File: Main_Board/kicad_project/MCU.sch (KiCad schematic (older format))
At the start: 35 parts

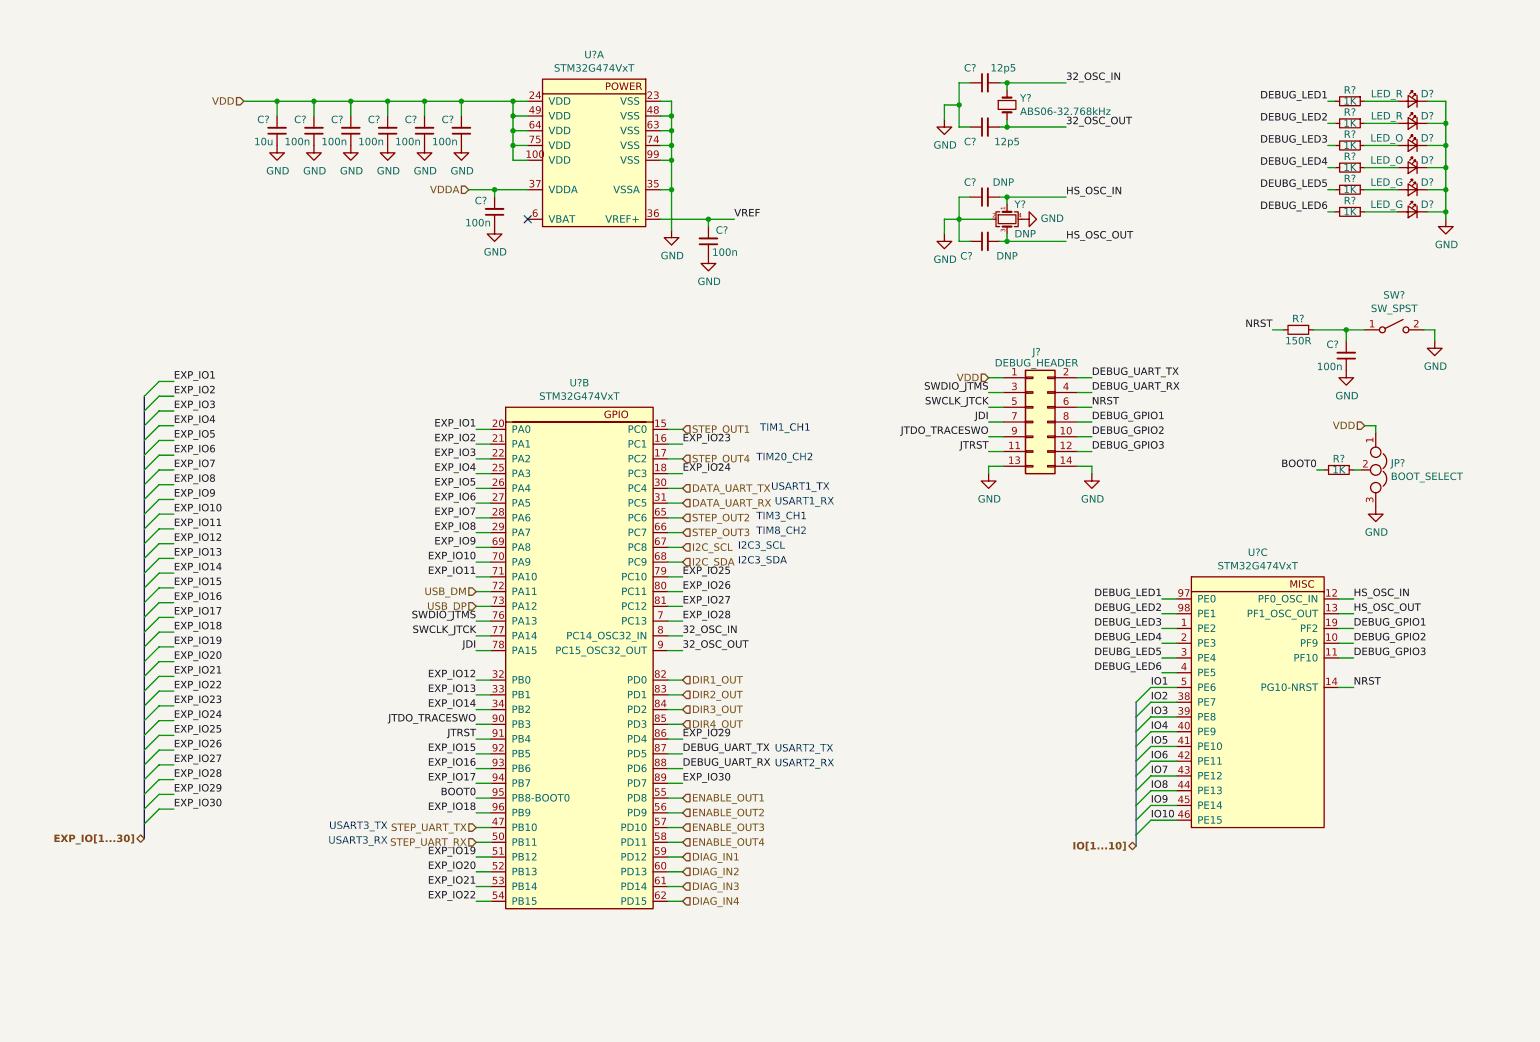
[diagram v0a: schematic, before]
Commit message: schematic rev1 finished
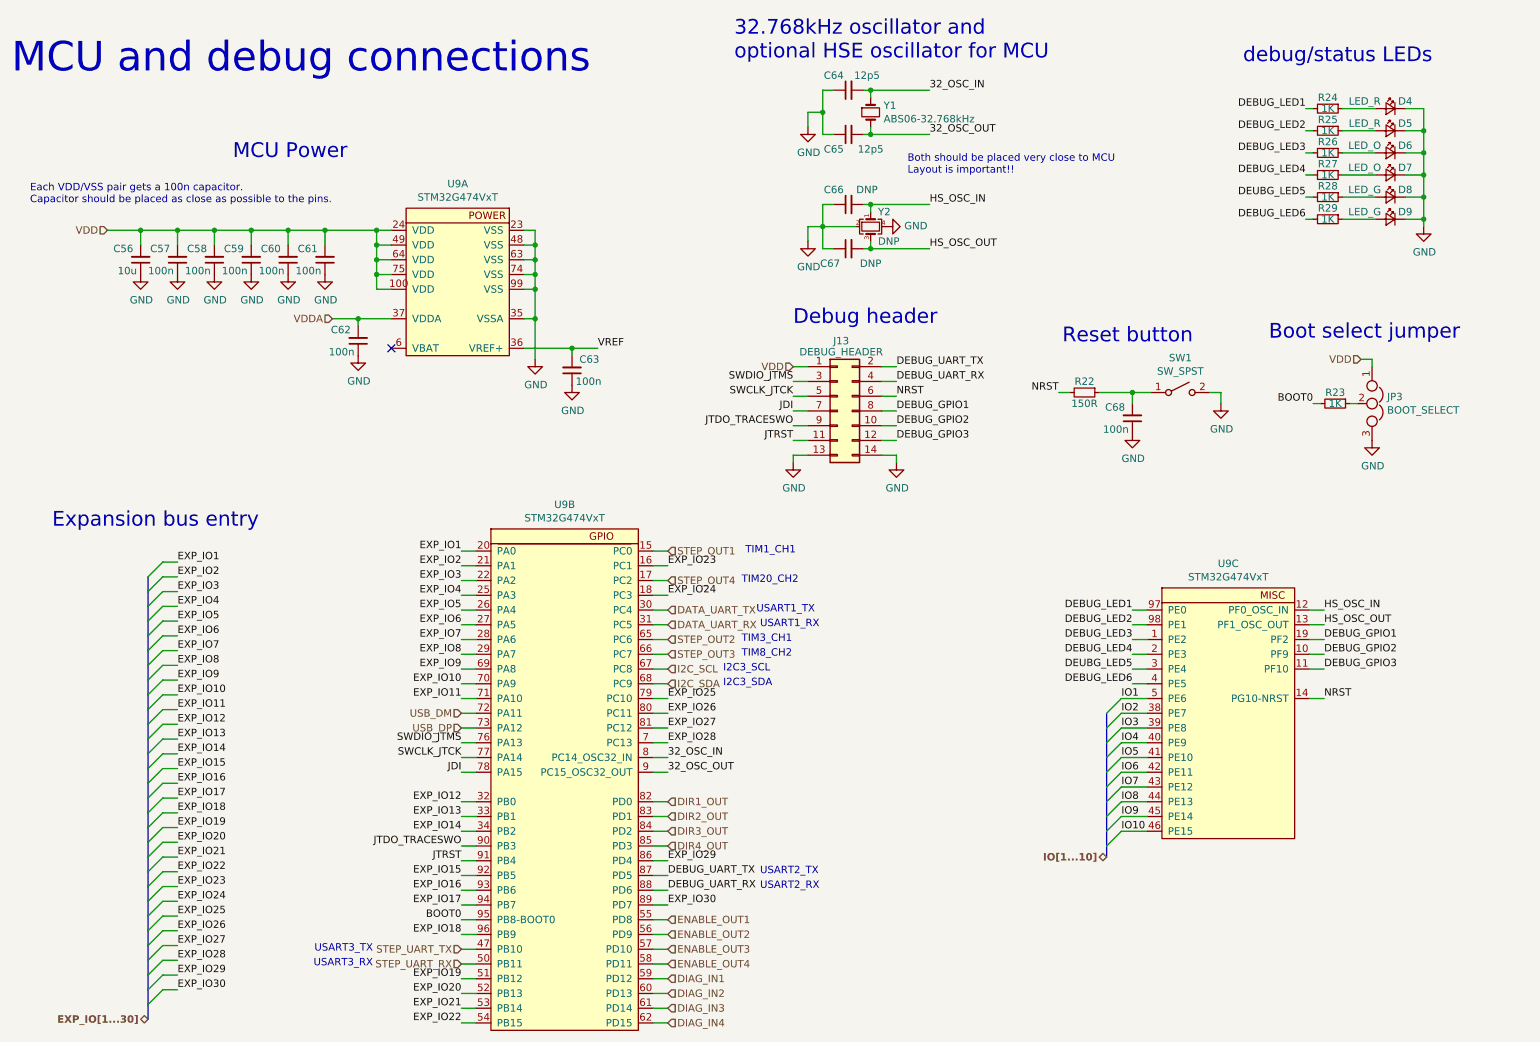
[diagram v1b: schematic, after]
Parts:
- gave numbers to parts that had none: 33
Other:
- note added: "32.768kHz oscillator and\noptional HSE oscillator for MCU"
- note added: "Boot select jumper"
- note added: "Both should be placed very close to MCU\nLayout is important!!"
- note added: "Debug header"
- note added: "Each VDD/VSS pair gets a 100n capacitor.\nCapacitor should be placed as close as possible to the pins."
- note added: "Expansion bus entry"
- note added: "MCU Power"
- note added: "MCU and debug connections"
- note added: "Reset button"
- note added: "debug/status LEDs"
- moved on the sheet: C56, C57, C58, C59, C60, C61, C62, C63, C64, C65, C66, C67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
